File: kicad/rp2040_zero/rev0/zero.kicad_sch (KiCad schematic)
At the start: 13 parts, among them J1 jtag, J2 Conn_01x03_Socket, J5 Debug port, U1 RP2040-Zero, U3 3V->VTREF, U4 VTREF->3V, U5 VTREF<->3V, U6 RT9013-33GB

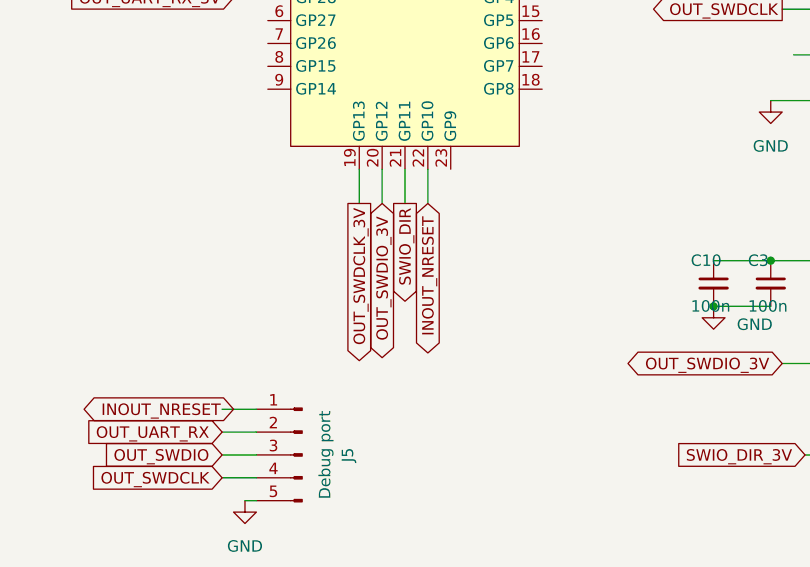
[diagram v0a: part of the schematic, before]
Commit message: RP2040: Carrier board
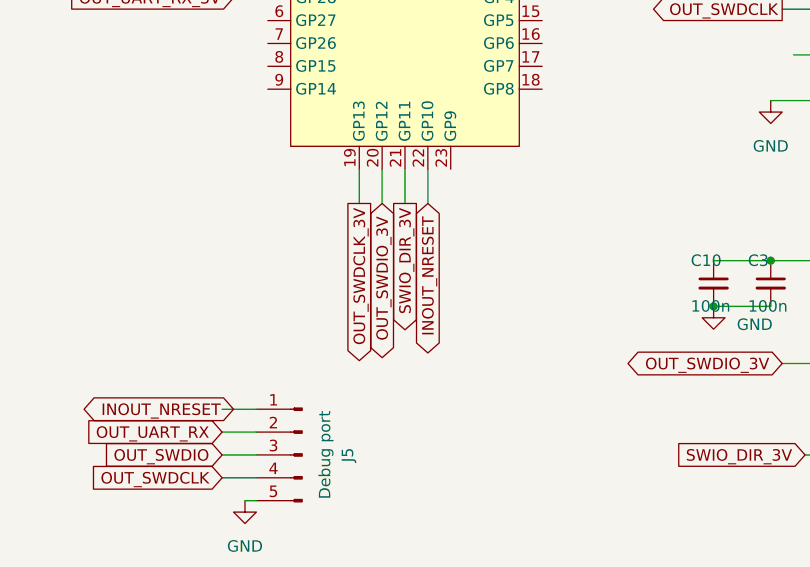
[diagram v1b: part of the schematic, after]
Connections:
- net SWIO_DIR is gone; now on net SWIO_DIR_3V: U1.21 (GP11)
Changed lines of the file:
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@@
 		)
 	)
-	(global_label "SWIO_DIR"
+	(global_label "SWIO_DIR_3V"
 		(shape output)
 		(at 55.88 63.5 270)
@@
 		)
 		(property "Intersheetrefs" "${INTERSHEET_REFS}"
-			(at 55.88 75.1938 90)
+			(at 55.88 78.4595 90)
 			(effects
 				(font

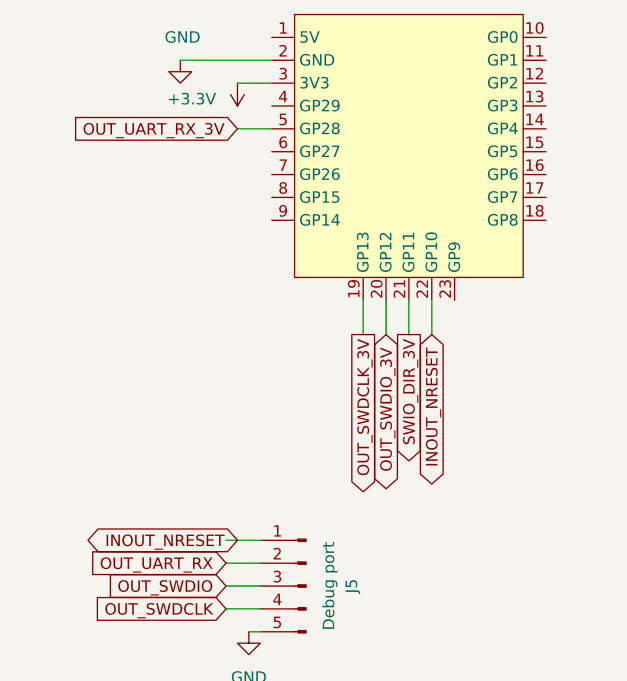
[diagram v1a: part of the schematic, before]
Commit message: cleanup
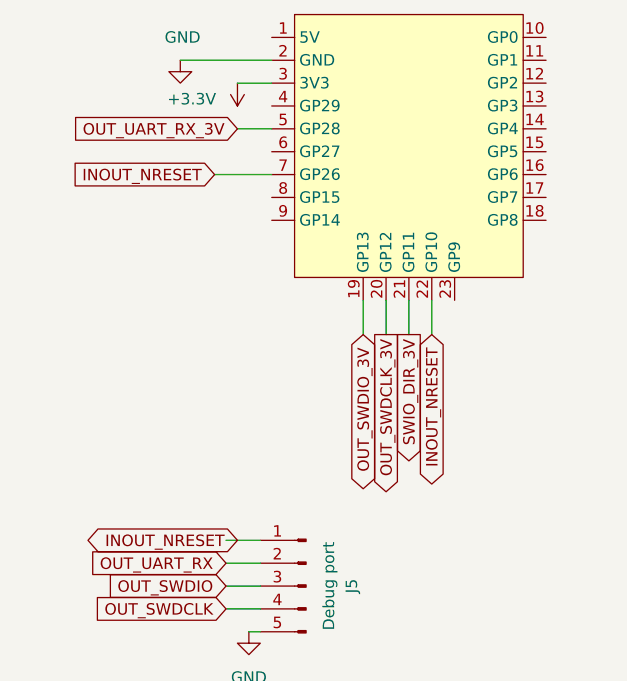
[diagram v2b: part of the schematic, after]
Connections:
- net INOUT_NRESET: now also U1.7 (GP26)
- net OUT_SWDCLK_3V: now also U1.20 (GP12); no longer U1.19 (GP13)
- net OUT_SWDIO_3V: now also U1.19 (GP13); no longer U1.20 (GP12)
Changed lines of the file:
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@@
+	(wire
+		(pts
+			(xy 34.29 45.72) (xy 40.64 45.72)
+		)
+		(stroke
+			(width 0)
+			(type default)
+		)
+	)
 	(wire
 		(pts
@@
 			(width 0)
 			(type default)
+		)
+	)
+	(global_label "INOUT_NRESET"
+		(shape input)
+		(at 34.29 45.72 180)
+		(fields_autoplaced yes)
+		(effects
+			(font
+				(size 1.27 1.27)
+			)
+			(justify right)
+		)
+		(property "Intersheetrefs" "${INTERSHEET_REFS}"
+			(at 17.6977 45.72 0)
+			(effects
+				(font
+					(size 1.27 1.27)
+				)
+				(justify right)
+				(hide yes)
+			)
 		)
 	)
@@
 	(global_label "OUT_SWDCLK_3V"
 		(shape output)
-		(at 50.8 63.5 270)
-		(fields_autoplaced yes)
-		(effects
-			(font
-				(size 1.27 1.27)
-			)
-			(justify right)
-		)
-		(property "Intersheetrefs" "${INTERSHEET_REFS}"
-			(at 50.8 81.8461 90)
+		(at 53.34 63.5 270)
+		(fields_autoplaced yes)
+		(effects
+			(font
+				(size 1.27 1.27)
+			)
+			(justify right)
+		)
+		(property "Intersheetrefs" "${INTERSHEET_REFS}"
+			(at 53.34 81.8461 90)
 			(effects
 				(font
@@
 	(global_label "OUT_SWDIO_3V"
 		(shape bidirectional)
-		(at 53.34 63.5 270)
-		(fields_autoplaced yes)
-		(effects
-			(font
-				(size 1.27 1.27)
-			)
-			(justify right)
-		)
-		(property "Intersheetrefs" "${INTERSHEET_REFS}"
-			(at 53.34 81.3246 90)
-			(effects
-				(font
+		(at 50.8 63.5 270)
+		(fields_autoplaced yes)
+		(effects
+			(font
+				(size 1.27 1.27)
+			)
+			(justify right)
+		)
+		(property "Intersheetrefs" "${INTERSHEET_REFS}"
+			(at 50.8 81.3246 90)
+			(effects
+				(font
